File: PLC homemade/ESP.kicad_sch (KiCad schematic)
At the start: 1 part, among them U9 ESP32-S3-WROOM-1U-N16R8

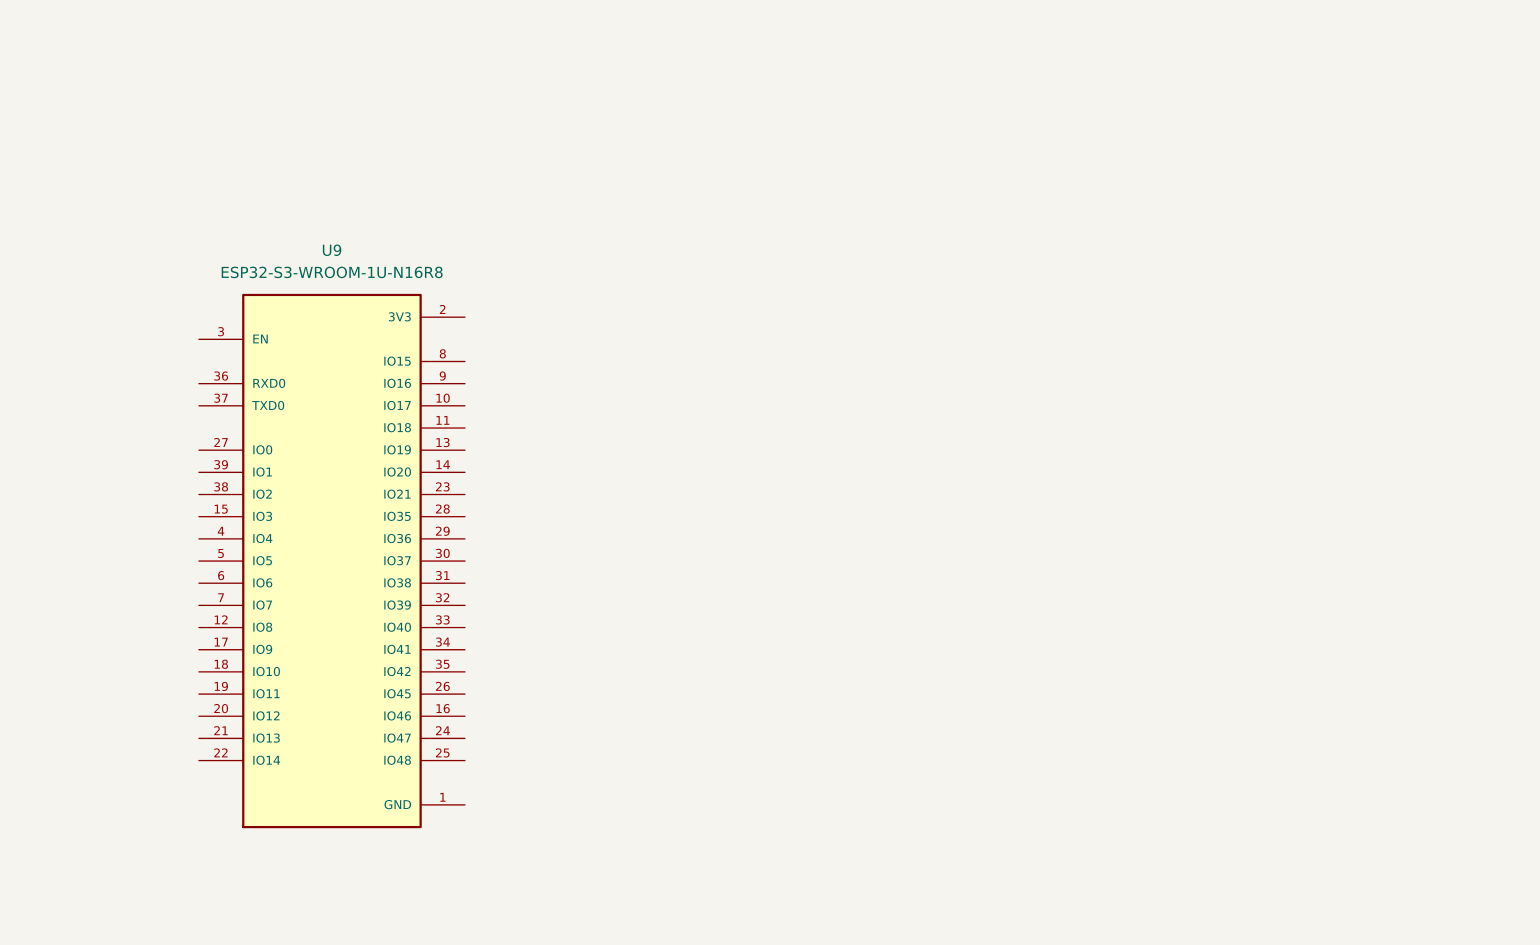
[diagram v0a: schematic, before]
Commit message: ::construction_worker:: Completed esp
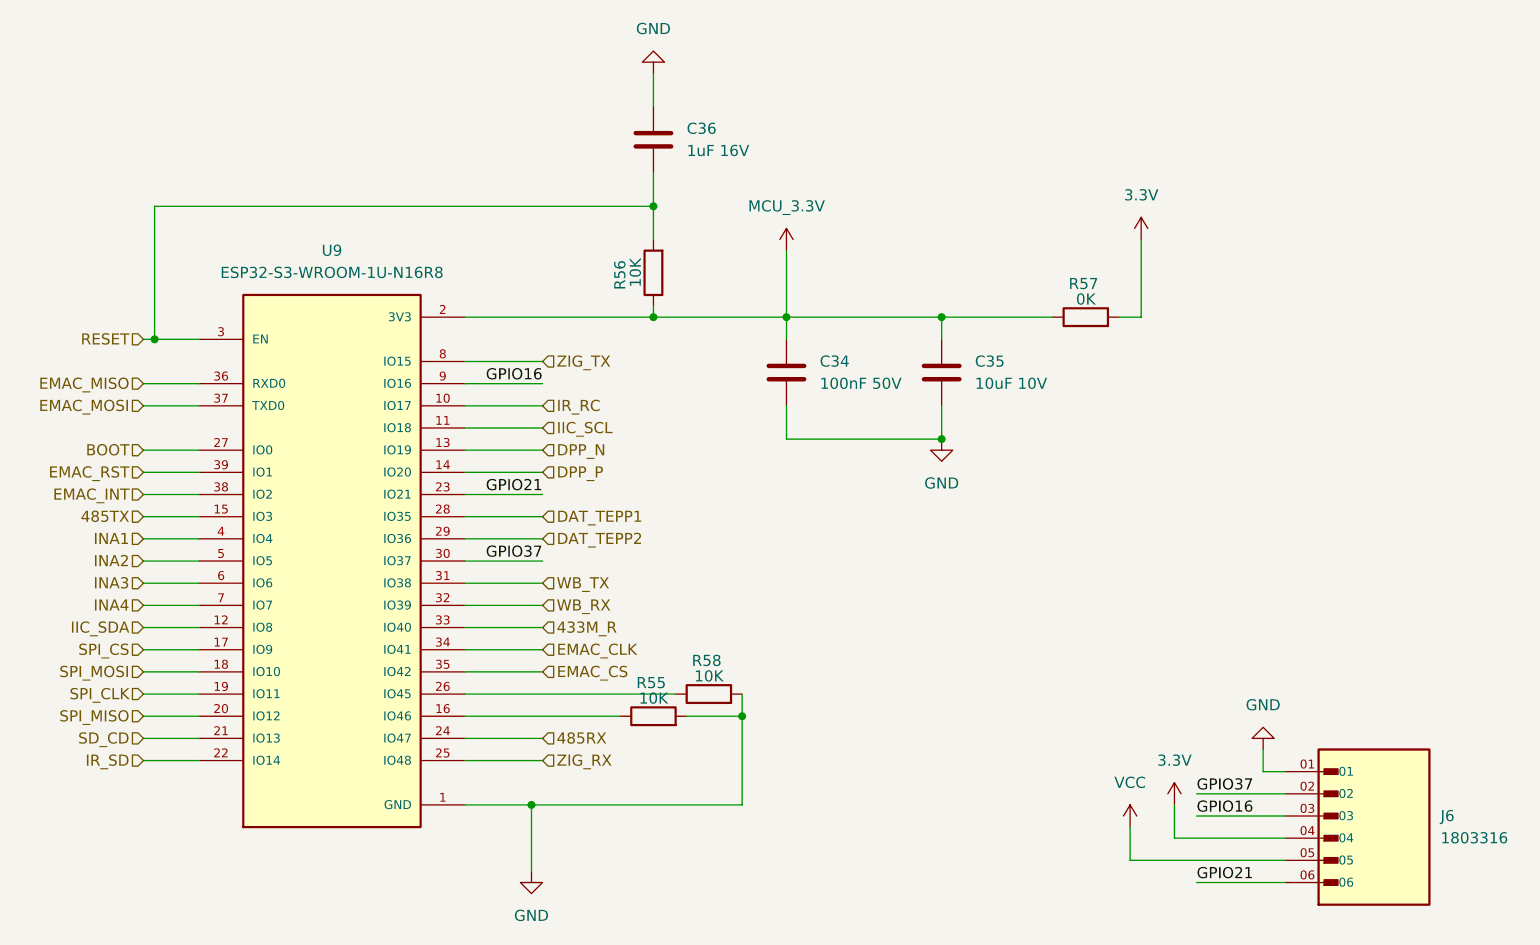
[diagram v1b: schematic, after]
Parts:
- added C34: 100nF 50V, symbol Device:C
- added C35: 10uF 10V, symbol Device:C
- added C36: 1uF 16V, symbol Device:C
- added J6: 1803316, 1803316:PHOENIX_1803316, symbol 1803316:1803316
- added R55, R56, R58: 10K, symbol Device:R
- added R57: 0K, symbol Device:R
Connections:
- net GND: now also C34.2, C35.2, C36.1, J6.01, R55.2, R58.2
- net IR_RC: now reaches U9.10 (IO17)
- net IIC_SCL: now reaches U9.11 (IO18)
- net IIC_SDA: now reaches U9.12 (IO8)
- net DPP_N: now reaches U9.13 (IO19)
- net DPP_P: now reaches U9.14 (IO20)
- net 485TX: now reaches U9.15 (IO3)
- net at U9.16 (IO46): now also R55.1
- net SPI_CS: now reaches U9.17 (IO9)
- net SPI_MOSI: now reaches U9.18 (IO10)
- net SPI_CLK: now reaches U9.19 (IO11)
- net MCU_3.3V: now reaches U9.2 (3V3)
- net MCU_3.3V: now also C34.1, C35.1, R56.1, R57.1
- net SPI_MISO: now reaches U9.20 (IO12)
- net SD_CD: now reaches U9.21 (IO13)
- net IR_SD: now reaches U9.22 (IO14)
- net GPIO21: now reaches U9.23 (IO21)
- net GPIO21: now also J6.06
- net 485RX: now reaches U9.24 (IO47)
- net ZIG_RX: now reaches U9.25 (IO48)
- net at U9.26 (IO45): now also R58.1
- net BOOT: now reaches U9.27 (IO0)
- net DAT_TEPP1: now reaches U9.28 (IO35)
- net DAT_TEPP2: now reaches U9.29 (IO36)
- net RESET: now reaches U9.3 (EN)
- net RESET: now also C36.2, R56.2
- net GPIO37: now reaches U9.30 (IO37)
- net GPIO37: now also J6.02
- net WB_TX: now reaches U9.31 (IO38)
- net WB_RX: now reaches U9.32 (IO39)
- net 433M_R: now reaches U9.33 (IO40)
- net EMAC_CLK: now reaches U9.34 (IO41)
- net EMAC_CS: now reaches U9.35 (IO42)
- net EMAC_MISO: now reaches U9.36 (RXD0)
- net EMAC_MOSI: now reaches U9.37 (TXD0)
- net EMAC_INT: now reaches U9.38 (IO2)
- net EMAC_RST: now reaches U9.39 (IO1)
- net INA1: now reaches U9.4 (IO4)
- net INA2: now reaches U9.5 (IO5)
- net INA3: now reaches U9.6 (IO6)
- net INA4: now reaches U9.7 (IO7)
- net ZIG_TX: now reaches U9.8 (IO15)
- net GPIO16: now reaches U9.9 (IO16)
- net GPIO16: now also J6.03
- new net 3.3V: J6.04, R57.2
- new net VCC: J6.05
